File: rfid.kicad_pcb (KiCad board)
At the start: 2 copper layers, 100 x 80 mm, 36 parts, among them U1 ATtiny25-20SS

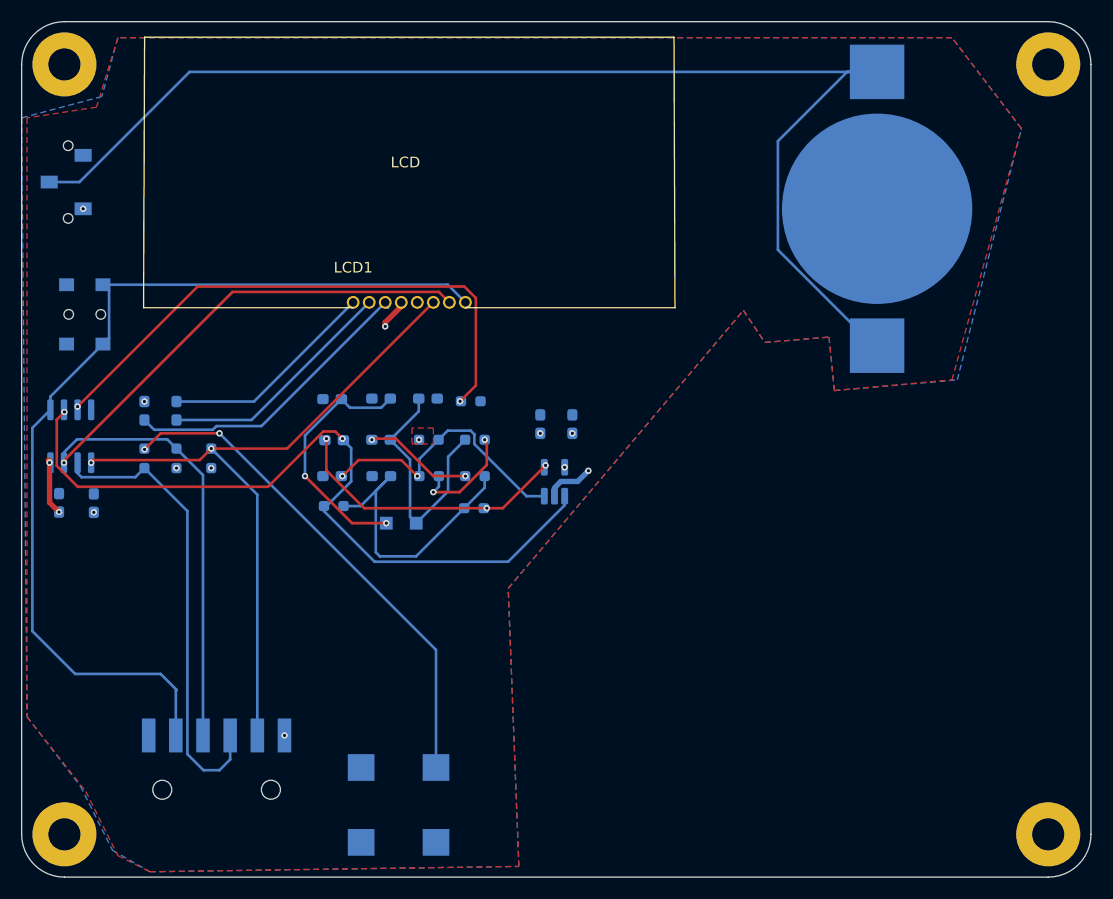
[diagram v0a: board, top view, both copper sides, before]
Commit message: New version
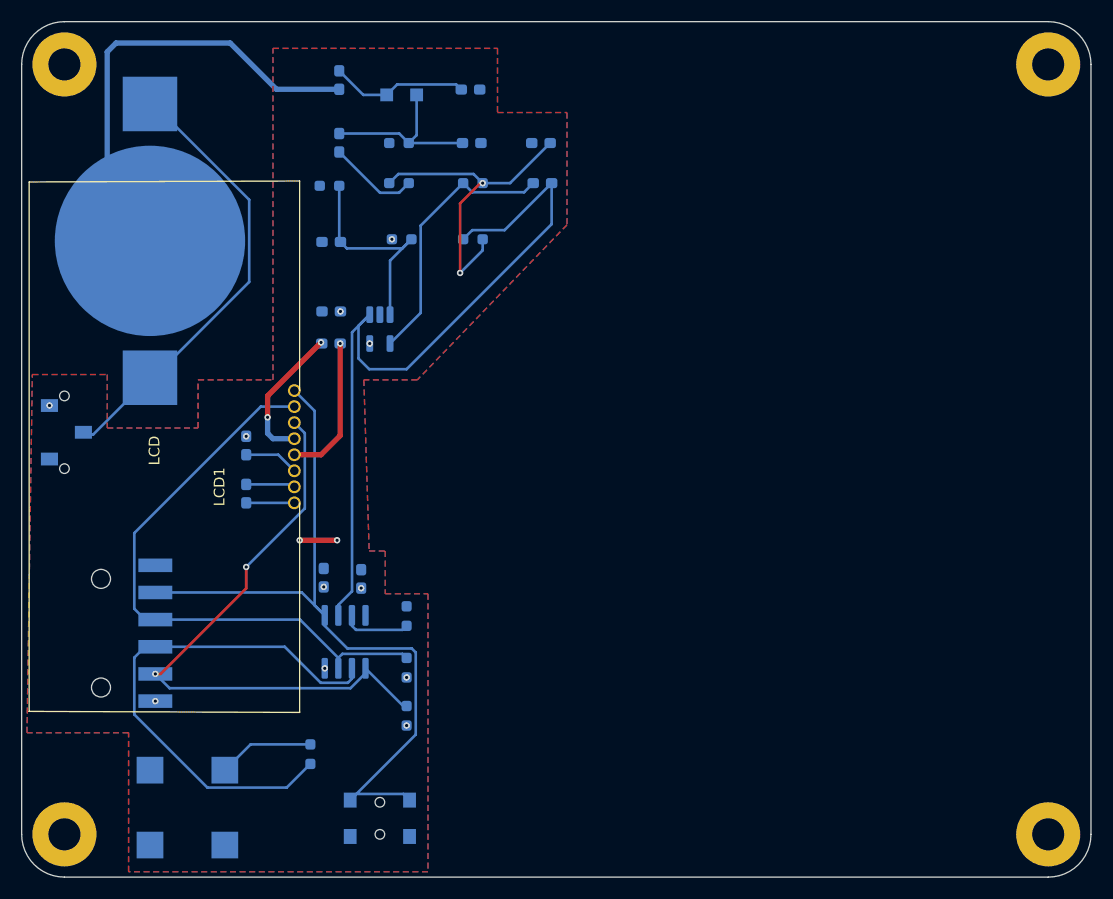
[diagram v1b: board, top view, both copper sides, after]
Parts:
- SW1: footprint X7:PowerSwitch -> X7:CL-SB-12A-11T
- moved BT1 68.1 mm to (25.5, 34.0)
- moved SW2 55.3 mm to (47.0, 88.5), turned to -90 degrees
- moved D1 40.1 mm to (49.0, 20.4)
- moved C4 34.5 mm to (62.1, 24.9)
- moved U1 32.1 mm to (43.8, 71.5)
- moved R8 31.7 mm to (40.5, 82.0)
- moved C5 30.9 mm to (62.2, 28.6)
- moved R4 30.4 mm to (55.7, 28.6), turned to 0 degrees
- moved R10 30.2 mm to (49.5, 78.4)
- moved C1 30.1 mm to (55.5, 19.9), turned to 0 degrees
- moved C1A1 29.8 mm to (43.2, 19.0), turned to -90 degrees
- moved C7 29.1 mm to (45.2, 65.6)
- moved R9 29.1 mm to (49.5, 73.9)
- moved R7 28.7 mm to (42.3, 28.9), turned to 0 degrees
- moved R2 28.6 mm to (48.8, 24.9), turned to 0 degrees
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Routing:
- net Net-(BT1-Pad1): track 116.8 -> 42.6 mm
- net /RFOUT: track 53.1 -> 6.40 mm, vias 2 -> 0
- net GND: track 14.8 -> 60.2 mm, vias 3 -> 4
- net Net-(BZ1-Pad1): track 47.3 -> 9.00 mm, vias 2 -> 0
- net /SCL: track 83.4 -> 55.6 mm, vias 1 -> 0
- net Net-(LCD1-VOUT): track 29.1 -> 5.12 mm
- net Net-(LCD1-C+): track 22.6 -> 4.59 mm
- net /RST: track 90.3 -> 72.8 mm
- net Net-(LCD1-C-): track 20.4 -> 4.50 mm
- net /SDA: track 67.0 -> 56.5 mm
- net Net-(D1-A): track 23.3 -> 12.9 mm, vias 2 -> 0
- net Net-(D1-K): track 23.5 -> 16.7 mm
- net VCC: track 8.15 -> 13.6 mm, vias 13 -> 12
- net /BUZZER: track 43.4 -> 48.8 mm
- net VREF: track 25.8 -> 20.4 mm, vias 2 -> 0
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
